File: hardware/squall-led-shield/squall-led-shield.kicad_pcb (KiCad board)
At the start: 2 copper layers, 25.4 x 21 mm, 10 parts, among them J1 SQUALL_HEADER, Q1 Q_2NMOS

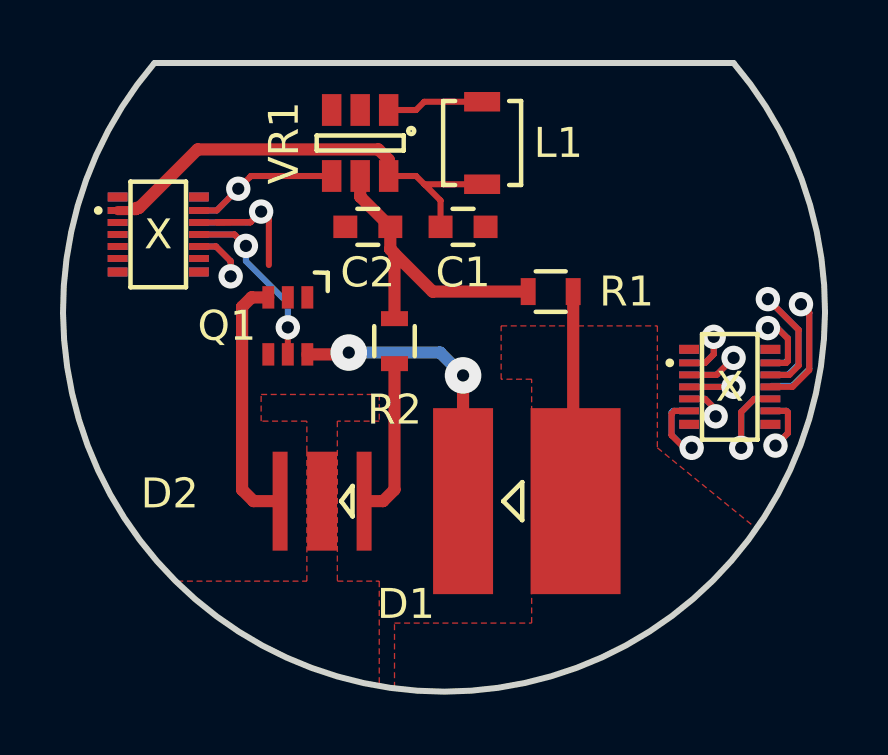
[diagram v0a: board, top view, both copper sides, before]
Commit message: Okay. That may be a board. Finally.
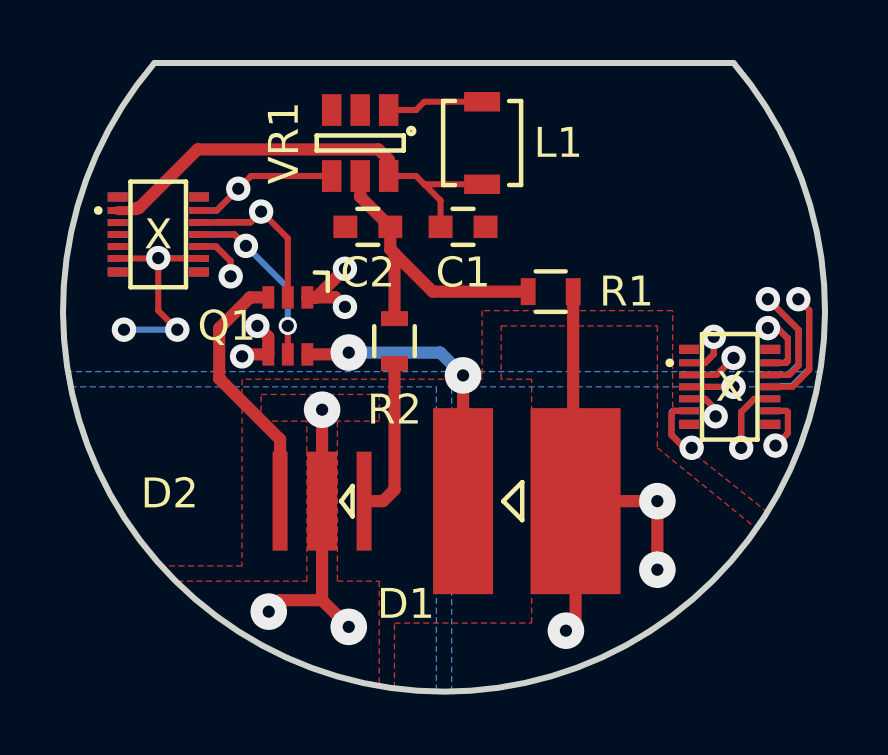
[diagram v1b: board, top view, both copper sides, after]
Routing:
- net GND: track 0.00 -> 13.5 mm, vias 0 -> 7
- net /CREE_THERMAL: track 0.00 -> 9.54 mm, vias 0 -> 3
- net Net-(D1-Pad2): track 7.02 -> 16.5 mm, vias 0 -> 3
- net /LED_IR: track 7.31 -> 8.65 mm
- added copper zone on B.Cu, net /CREE_THERMAL
- added copper zone on B.Cu, net GND
- added copper zone on F.Cu, net GND
- added copper zone on B.Cu, net Net-(D1-Pad2)
